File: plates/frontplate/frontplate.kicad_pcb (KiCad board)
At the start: 2 copper layers, 33.2 x 81.9 mm, 2 parts

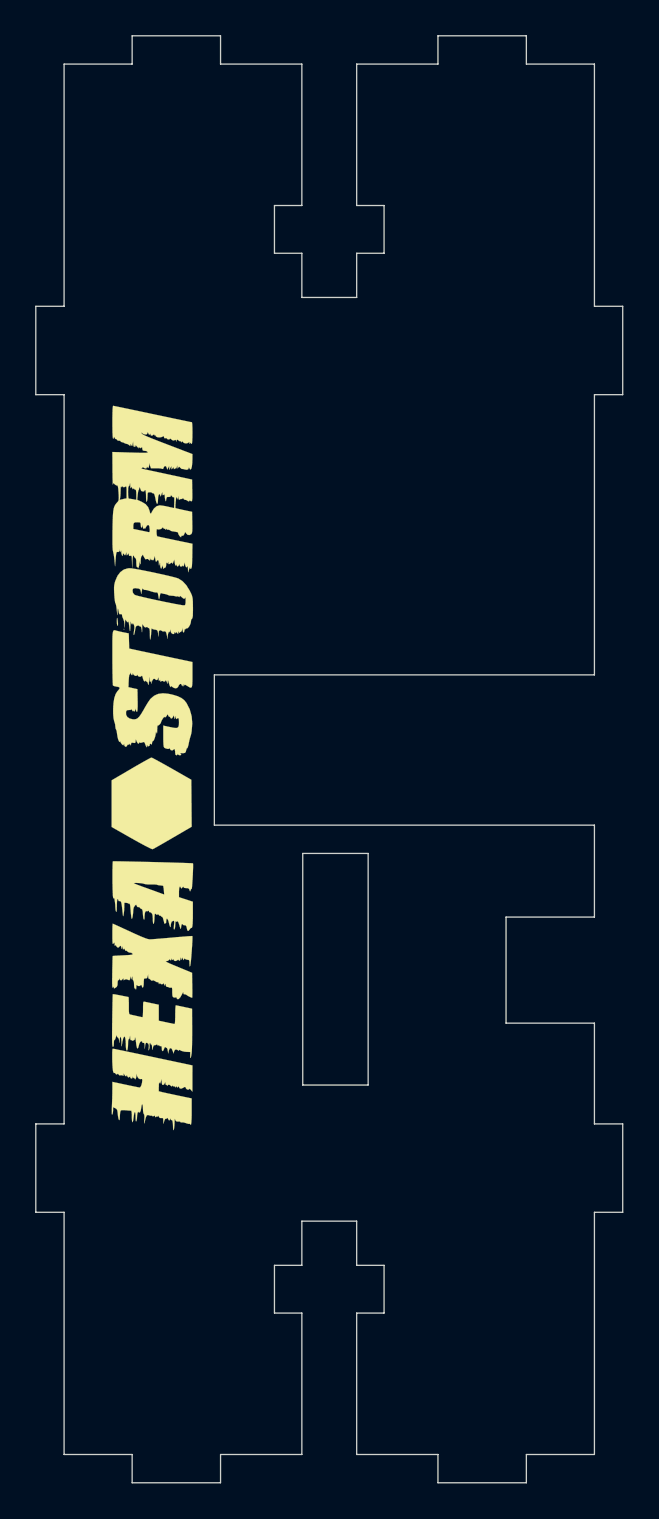
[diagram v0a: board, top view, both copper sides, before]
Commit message: added design of june
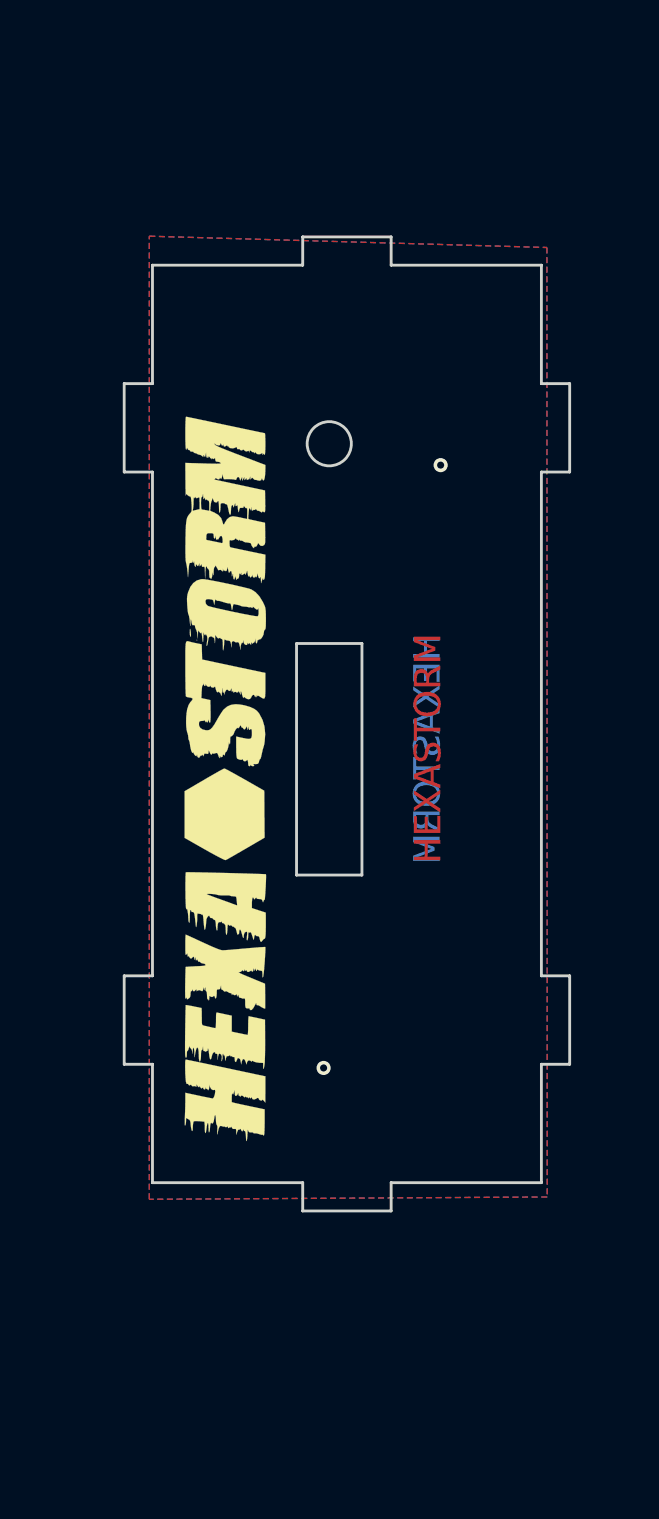
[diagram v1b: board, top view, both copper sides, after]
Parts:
- moved L2 4.29 mm to (148.2, 104.1)
- moved L1 4.17 mm to (148.2, 105.1)
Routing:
- net (no net): vias 0 -> 2
- added copper zone on B.Cu, net (none)
- added copper zone on F.Cu, net (none)
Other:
- board size 33.2 x 81.9 mm -> 25.2 x 55.1 mm
- net class Default removed
- board text added: "HEXASTORM"
